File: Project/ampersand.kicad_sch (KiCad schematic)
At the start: 19 parts, among them J1 JST SH, U1 STM32F072CBT6

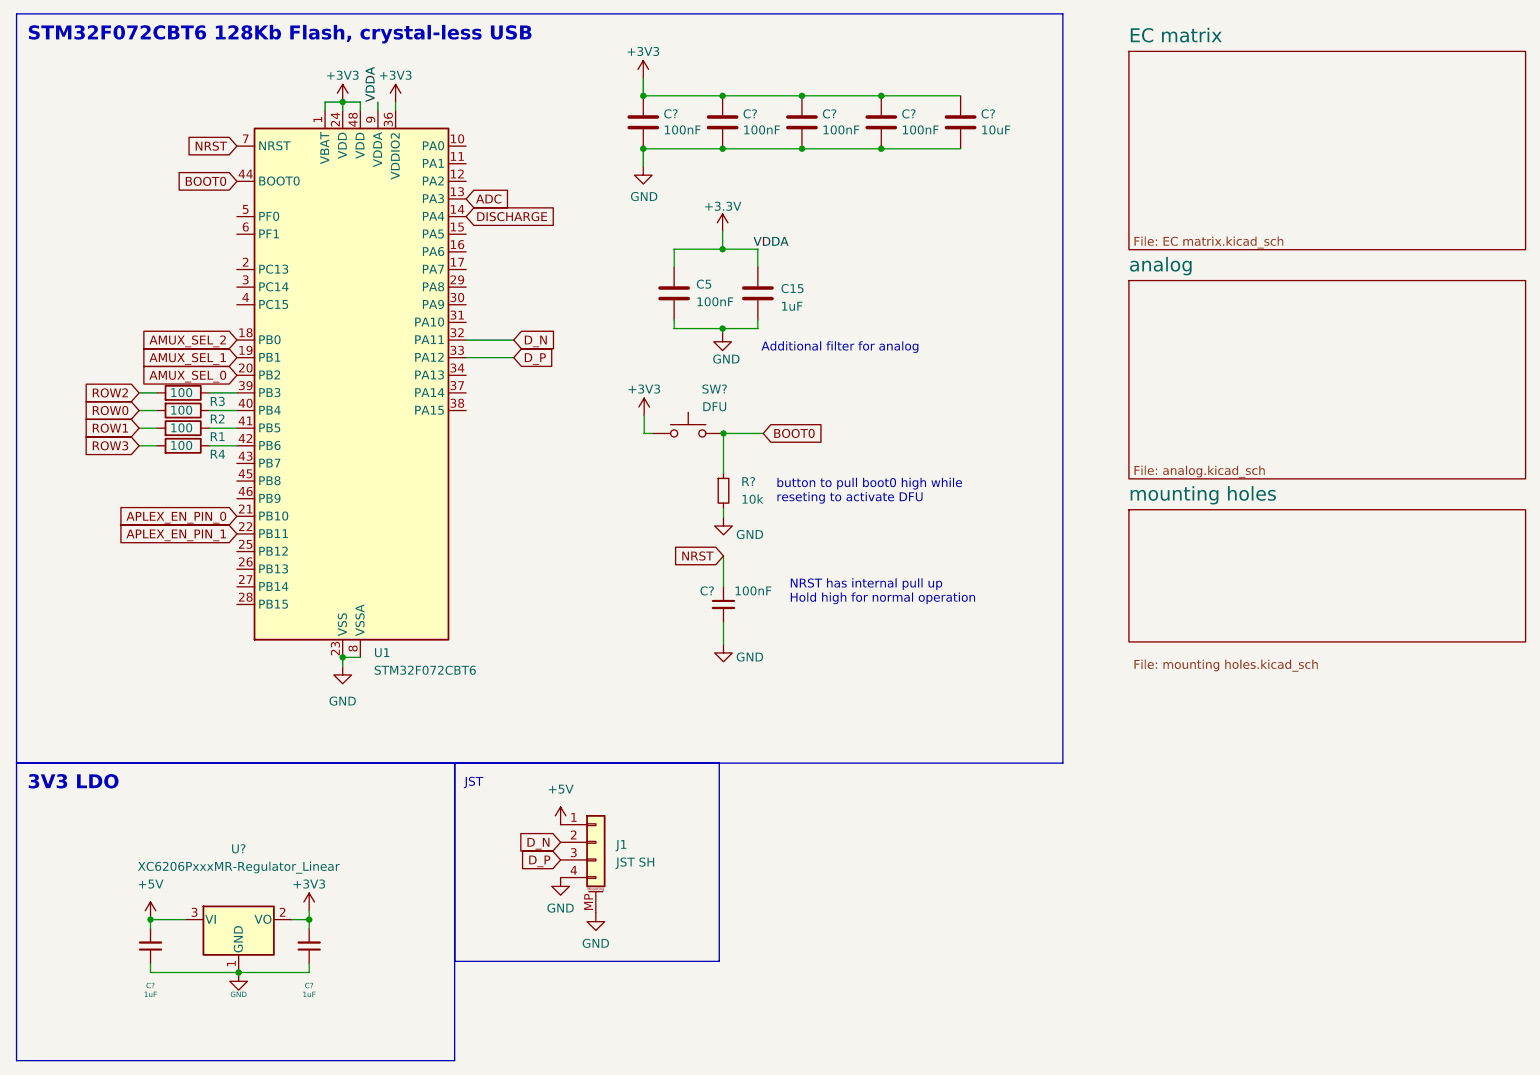
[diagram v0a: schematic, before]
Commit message: update & backup
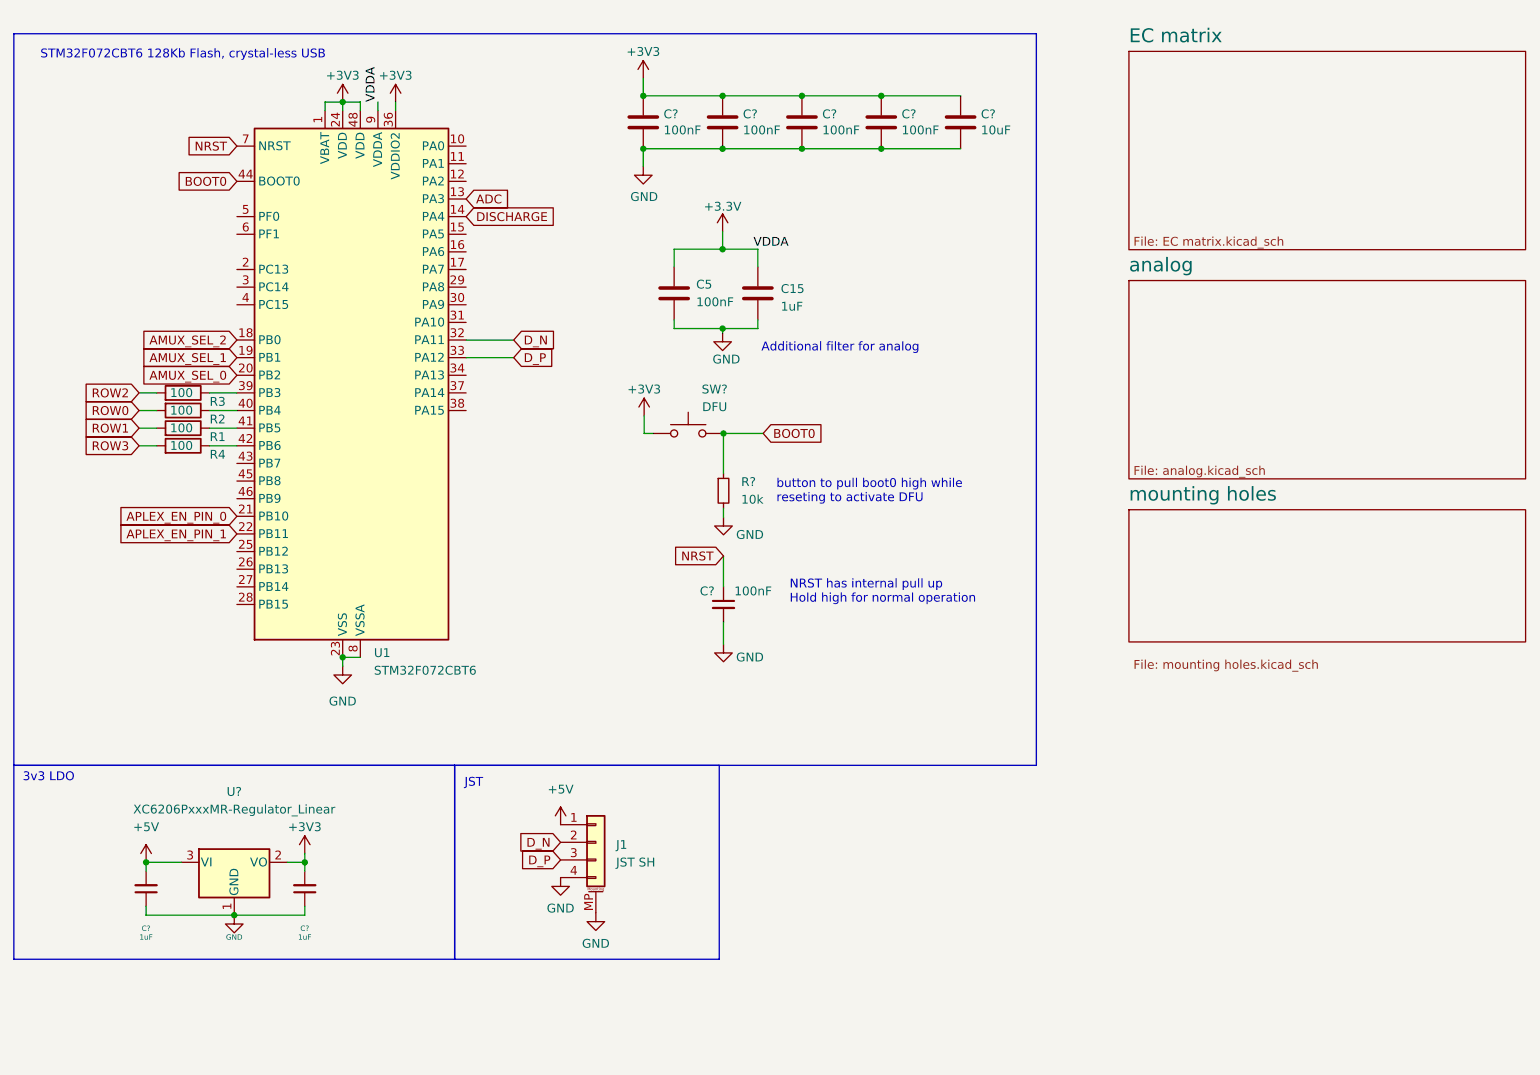
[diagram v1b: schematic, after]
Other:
- note added: "3v3 LDO"
- note added: "STM32F072CBT6 128Kb Flash, crystal-less USB"
- moved on the sheet: C?, U?

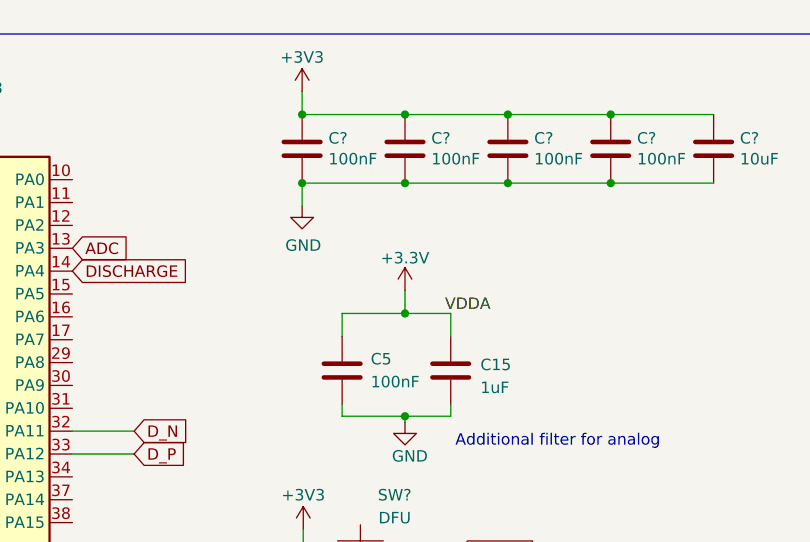
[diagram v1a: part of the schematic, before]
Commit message: v1 production files
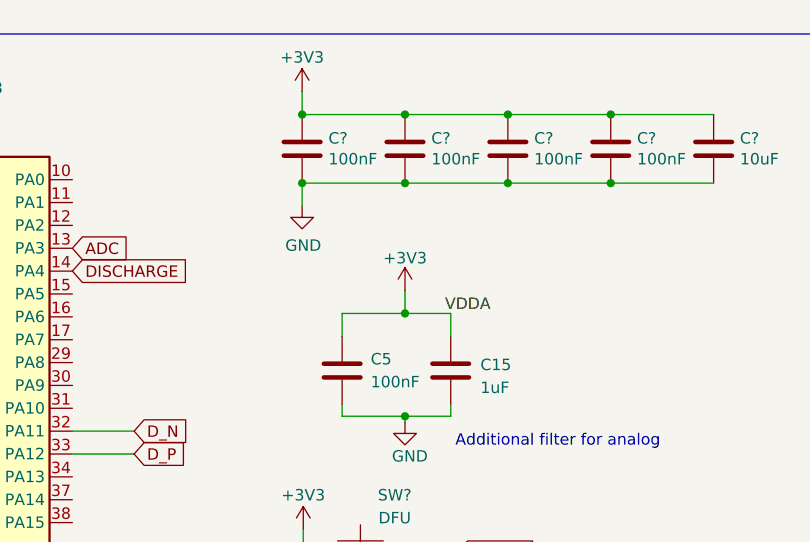
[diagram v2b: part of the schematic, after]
